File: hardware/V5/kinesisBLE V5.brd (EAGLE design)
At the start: 122 x 86 mm, 29 parts, among them X1 JST-XH-02-PIN-ROUND-PAD, X2 JST-XH-02-PIN-ROUND-PAD

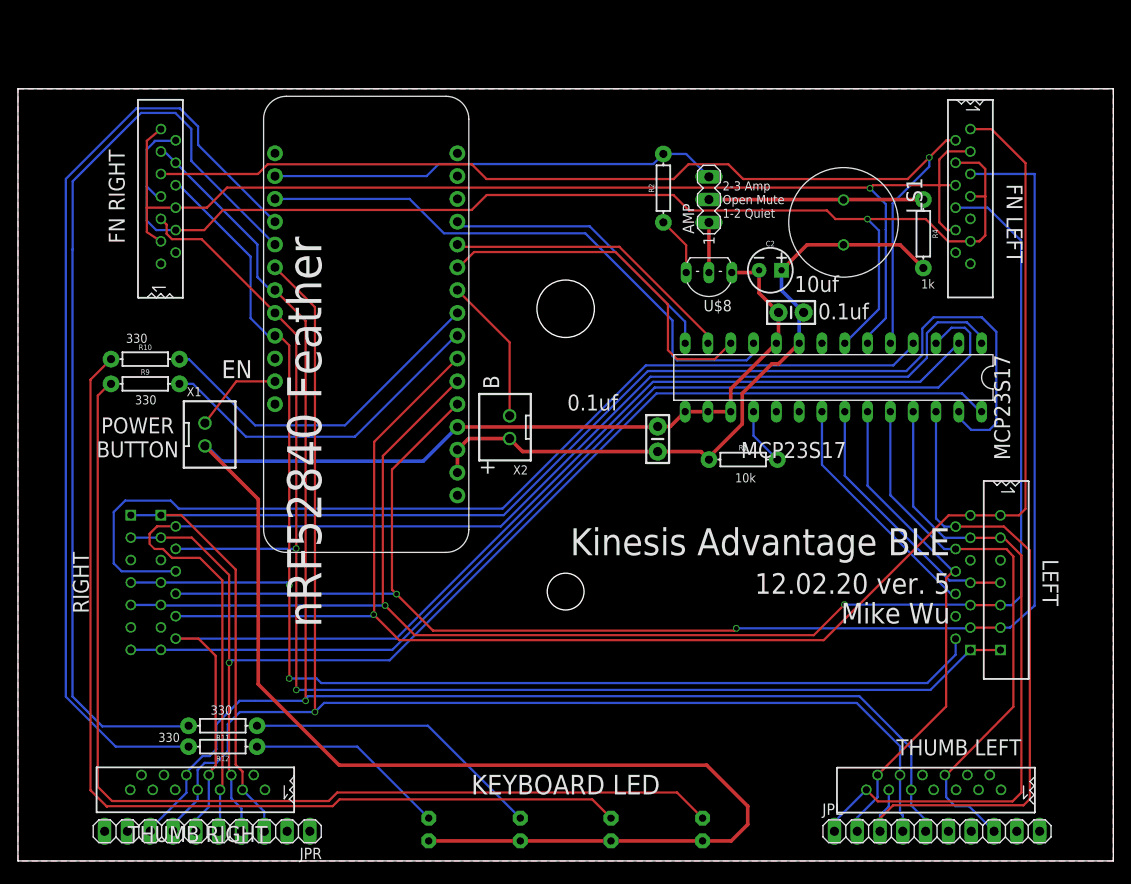
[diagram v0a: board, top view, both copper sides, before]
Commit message: submit
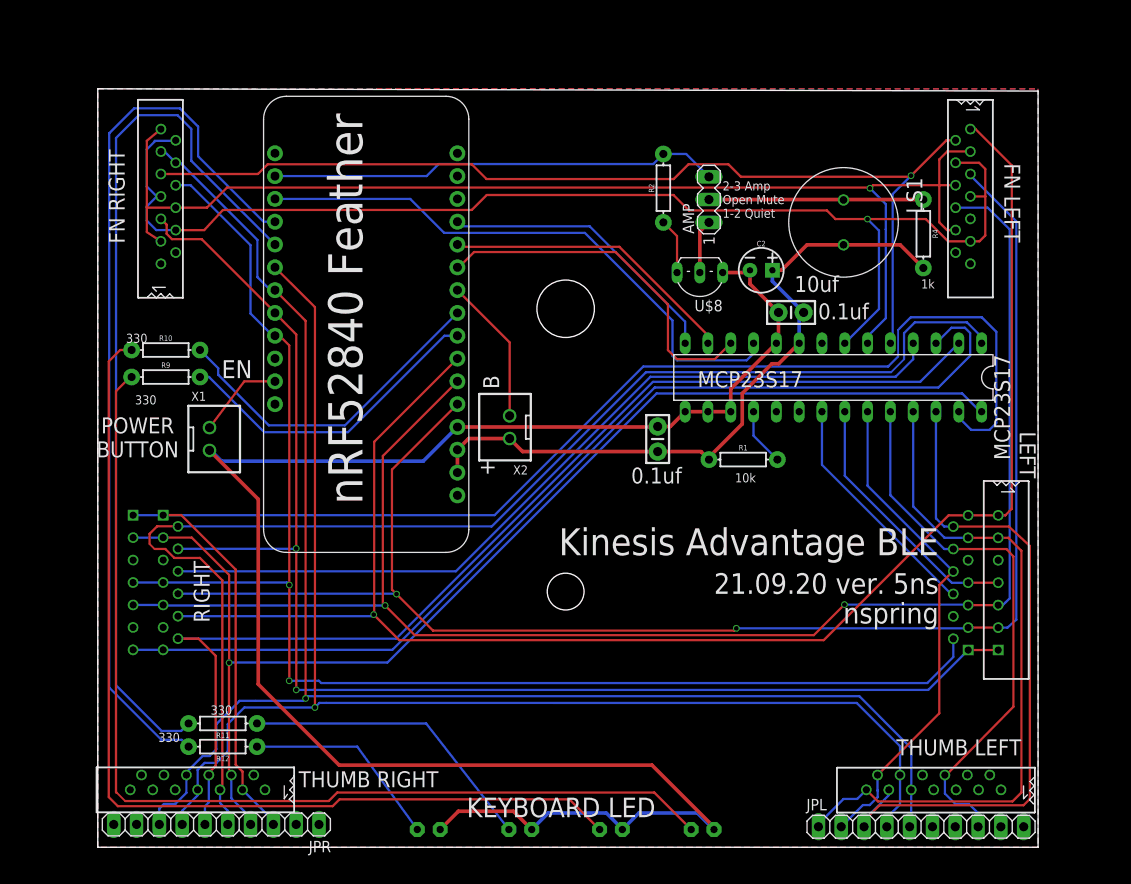
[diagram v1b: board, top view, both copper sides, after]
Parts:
- moved R10 2.50 mm to (16.5, 56.9)
- moved R9 2.41 mm to (16.5, 53.9)
- moved JPL 1.85 mm to (100.6, 3.81)
- moved JPR 1.27 mm to (22.1, 4.06)
- moved C2 1.02 mm to (82.8, 65.8)
- moved U$8 1.02 mm to (75.9, 65.5)
- moved X1 0.72 mm to (21.3, 47.0)
- moved U$5 0.25 mm to (105.7, 31.0)
- moved R11 0.25 mm to (22.8, 15.3)
- moved U$4 0.25 mm to (16.3, 31.0)
- turned LED1 to 180 degrees
- turned LED2 to 180 degrees
- turned LED3 to 180 degrees
- turned LED4 to 180 degrees
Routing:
- net COL-L: track 110.7 -> 93.4 mm
- net SCR: track 105.6 -> 98.3 mm
- net KEY: track 106.6 -> 100.1 mm
- net ROW-3: track 178.0 -> 171.7 mm
- net GND: track 211.0 -> 204.7 mm
- net ROW-1: track 180.5 -> 177.1 mm
- net COL-M: track 115.3 -> 112.2 mm
- net CAPS: track 38.1 -> 35.7 mm
- net ROW-2: track 179.3 -> 177.4 mm
- net ROW-7: track 154.1 -> 152.3 mm
- net COL-J: track 126.6 -> 124.9 mm
- net COL-F: track 75.5 -> 77.1 mm
- net ROW-6: track 175.0 -> 173.3 mm
- net N$1: track 115.2 -> 113.6 mm
- net NUM: track 39.2 -> 37.8 mm
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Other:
- board size 122 x 86 mm -> 104.7 x 84.5 mm
- board text added: "21.09.20 ver. 5ns"
- board text added: "nspring"
- board text removed: "12.02.20 ver. 5"
- board text removed: "Mike Wu"
